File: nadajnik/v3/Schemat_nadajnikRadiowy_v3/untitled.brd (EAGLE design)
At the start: 73.6 x 78.4 mm, 15 parts, among them M1 ELECTRET_MICROPHON-WM-61B, T1 BF199

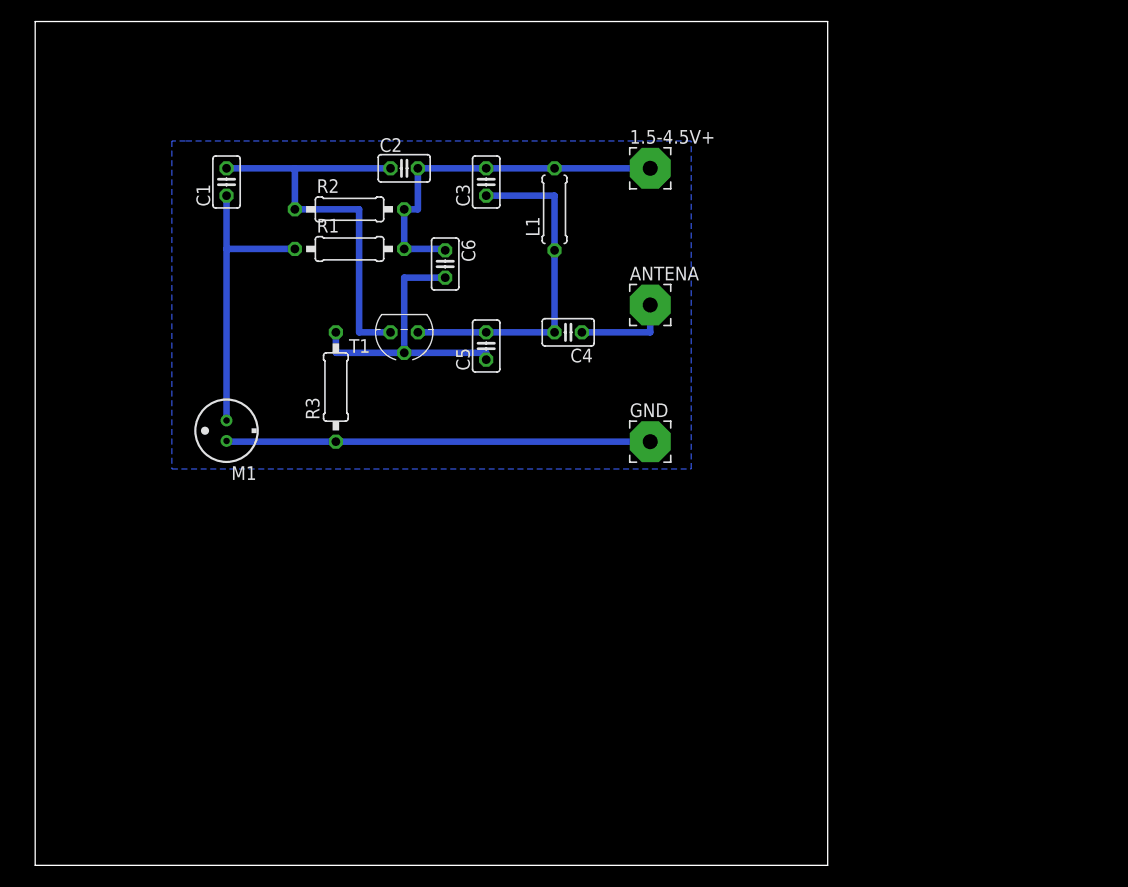
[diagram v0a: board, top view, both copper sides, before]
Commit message: nadajnik v3 plytka pcb
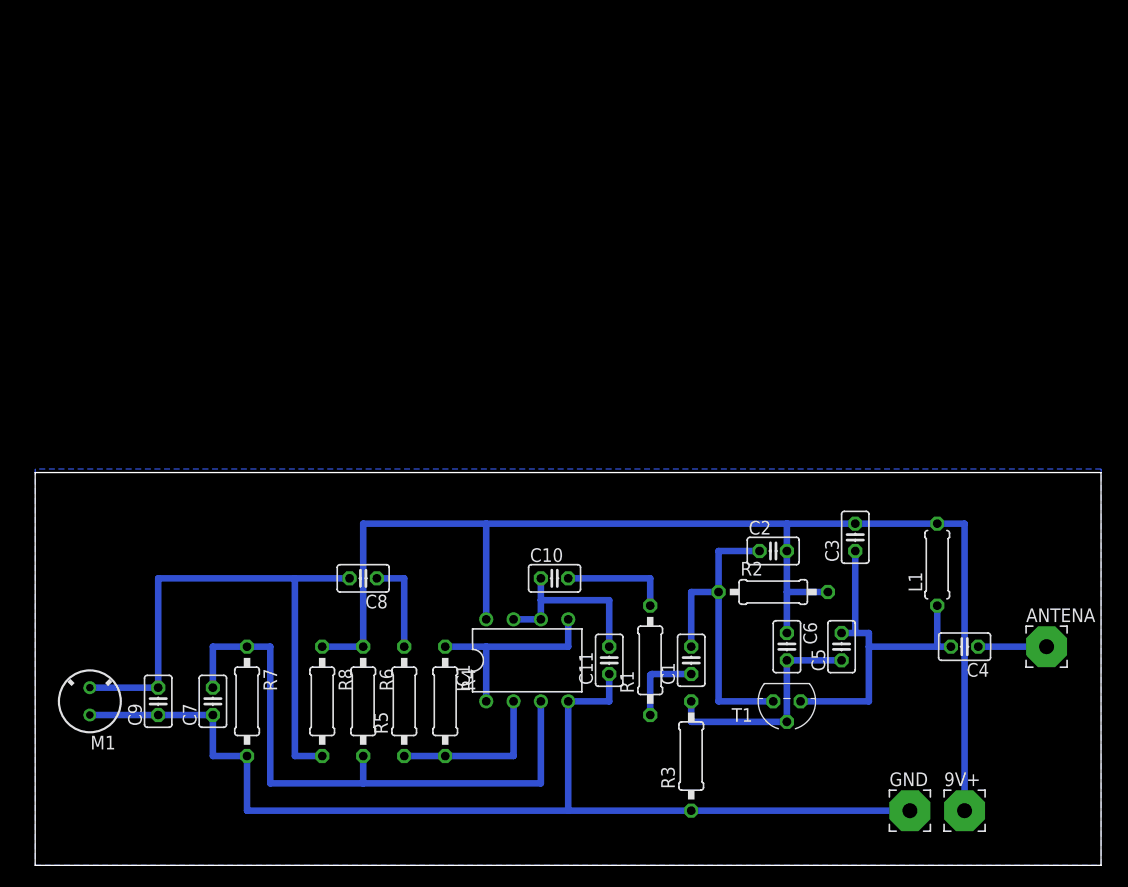
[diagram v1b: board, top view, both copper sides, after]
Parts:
- removed 1.5-4.5V+: (no value), wirepad:3,81/1,4
- added 9V+: (no value), wirepad:3,81/1,4
- added C10: 22u, rcl:C025-025X050
- added C11, C7, C9: 1n, rcl:C025-025X050
- added C8: 10u, rcl:C025-025X050
- added IC1: LM358N, linear:DIL08
- added R4: 150k, rcl:0207/10
- added R5: 300, rcl:0207/10
- added R6: 4.7k, rcl:0207/10
- added R7: 4.7, rcl:0207/10
- added R8: 1.8k, rcl:0207/10
- M1: value ELECTRET_MICROPHON-WM-61B -> ELECTRET_MICROPHON-F6050AP; device microphon:WM-61B -> microphon:F6050AP
- R1: value 1.8k -> 220
- moved C1 62.0 mm to (61.0, 19.1)
- moved R2 53.1 mm to (68.6, 25.4)
- moved C2 49.4 mm to (68.6, 29.2)
- moved T1 49.4 mm to (69.8, 15.2)
- moved ANTENA 48.6 mm to (94.0, 20.3)
- moved L1 48.5 mm to (83.8, 27.9)
- moved C6 47.7 mm to (69.8, 20.3)
- moved C3 47.6 mm to (76.2, 30.5)
- moved R3 47.6 mm to (61.0, 10.2)
- moved R1 47.3 mm to (57.1, 19.1), turned to 90 degrees
- moved C4 47.0 mm to (86.4, 20.3)
- moved C5 43.3 mm to (74.9, 20.3)
- moved GND 41.9 mm to (81.3, 5.08)
- moved M1 28.2 mm to (5.08, 15.2)
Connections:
- new net N$1: C10.2, R1.2
- new net N$10: IC1.2, R4.2, R5.1
- new net N$11: C7.2, IC1.3, R6.2, R7.1
- new net N$13: C8.1, R5.2
- new net N$14: C8.2, C9.2, M1.2, R8.2
- new net N$4: C10.1, C11.2, IC1.6, IC1.7
- new net N$9: IC1.1, IC1.5, R4.1
- net GND: now also C11.1, C7.1, C9.1, IC1.4, R7.2
- net N$2: no longer M1.2
- net N$7: now also 9V+.1, IC1.8, R6.1, R8.1; no longer 1.5-4.5V+.1, R1.2
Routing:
- net N$7: track 34.3 -> 120.8 mm
- net GND: track 39.4 -> 101.6 mm
- net N$11: track 0.00 -> 57.1 mm
- net N$14: track 0.00 -> 53.3 mm
- net N$2: track 27.2 -> 7.56 mm
- net N$9: track 0.00 -> 19.0 mm
- net N$4: track 0.00 -> 17.0 mm
- net N$10: track 0.00 -> 15.2 mm
- net N$1: track 0.00 -> 10.2 mm
- net N$3: track 39.4 -> 30.5 mm
- net N$13: track 0.00 -> 8.89 mm
- net N$5: track 27.3 -> 21.6 mm
- net N$6: track 31.7 -> 34.3 mm
- net N$8: track 8.89 -> 6.35 mm
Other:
- board size 73.6 x 78.4 mm -> 99 x 36.5 mm

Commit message: poprawa nadajnika
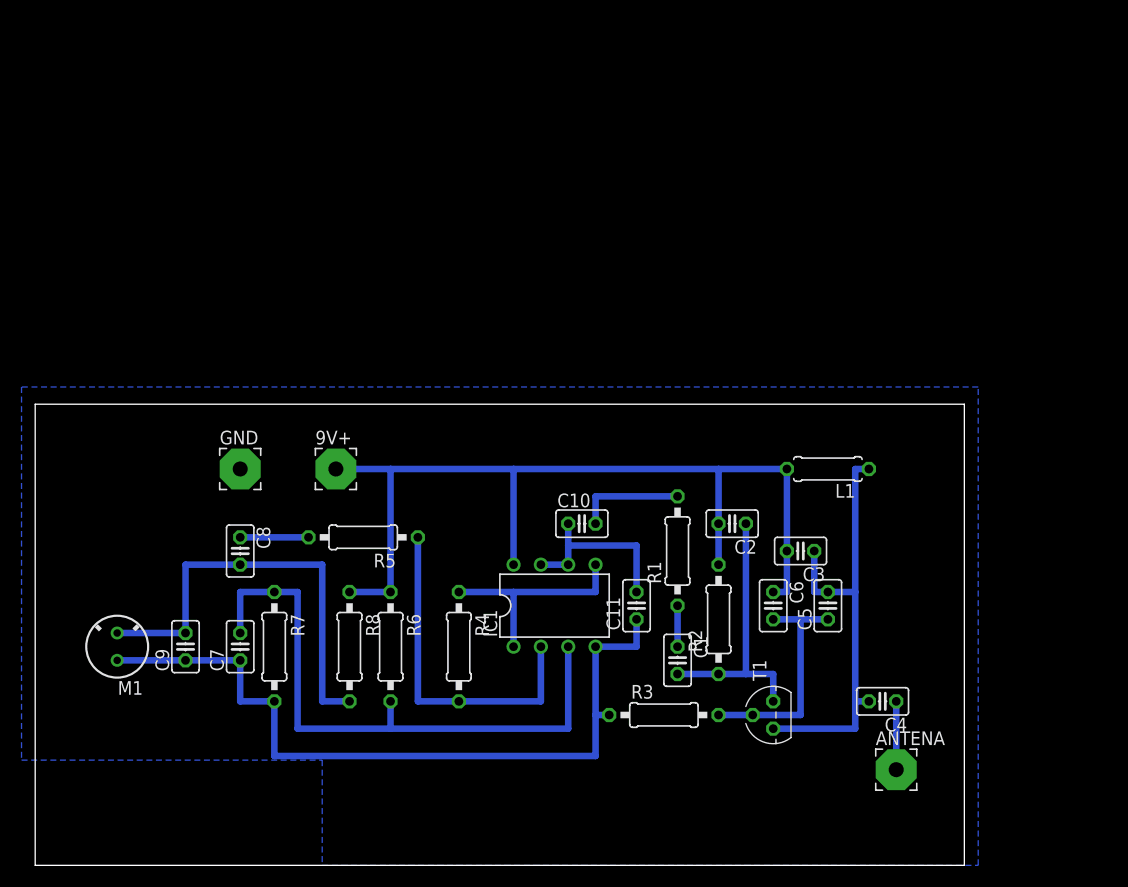
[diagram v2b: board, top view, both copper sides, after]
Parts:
- moved GND 69.9 mm to (19.1, 36.8)
- moved 9V+ 66.5 mm to (27.9, 36.8)
- moved ANTENA 18.1 mm to (80.0, 8.89)
- moved R5 15.7 mm to (30.5, 30.5), turned to 180 degrees
- moved L1 13.5 mm to (73.7, 36.8), turned to 180 degrees
- moved C8 11.7 mm to (19.1, 29.2), turned to 270 degrees
- moved R1 10.5 mm to (59.7, 29.2)
- moved C4 9.16 mm to (78.7, 15.2)
- moved R6 5.68 mm to (33.0, 20.3)
- moved R7 5.68 mm to (22.2, 20.3)
- moved C9 5.68 mm to (14.0, 20.3)
- moved M1 5.68 mm to (7.62, 20.3)
- moved C7 5.68 mm to (19.1, 20.3)
- moved R8 5.68 mm to (29.2, 20.3)
- moved C10 5.68 mm to (50.8, 31.8)
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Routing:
- net N$7: track 120.8 -> 87.6 mm
- net GND: track 101.6 -> 71.1 mm
- net N$10: track 15.2 -> 31.8 mm
- net N$14: track 53.3 -> 40.6 mm
- net N$6: track 34.3 -> 41.9 mm
- net N$3: track 30.5 -> 25.4 mm
- net N$2: track 7.56 -> 3.81 mm
- net N$13: track 8.89 -> 6.35 mm
- net N$9: track 19.0 -> 20.3 mm
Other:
- board size 99 x 36.5 mm -> 86.3 x 42.9 mm
- board text added: ""Siódemka" Mateusz Kitliński"
